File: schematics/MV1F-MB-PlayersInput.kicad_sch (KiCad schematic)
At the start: 55 parts

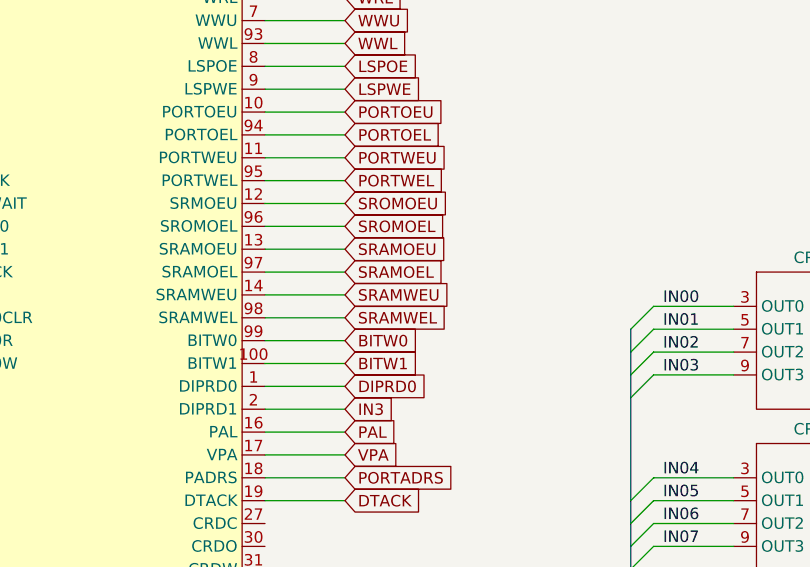
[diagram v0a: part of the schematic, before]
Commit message: Typo
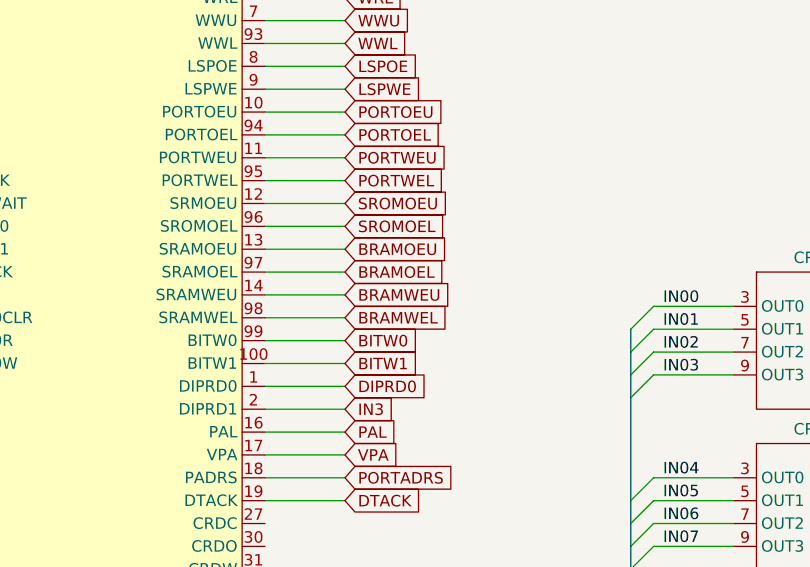
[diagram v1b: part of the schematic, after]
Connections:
- net SRAMOEL renamed BRAMOEL
- net SRAMOEU renamed BRAMOEU
- net SRAMWEL renamed BRAMWEL
- net SRAMWEU renamed BRAMWEU
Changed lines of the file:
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@@
     )
   )
-  (global_label "SRAMWEL" (shape input) (at 109.22 67.31 0) (fields_autoplaced)
-    (effects (font (size 1.27 1.27)) (justify left))
-    (property "Intersheetrefs" "${INTERSHEET_REFS}" (at 120.8532 67.31 0)
+  (global_label "BRAMWEL" (shape input) (at 109.22 67.31 0) (fields_autoplaced)
+    (effects (font (size 1.27 1.27)) (justify left))
+    (property "Intersheetrefs" "${INTERSHEET_REFS}" (at 120.9137 67.31 0)
       (effects (font (size 1.27 1.27)) (justify left))
     )
@@
     )
   )
-  (global_label "SRAMOEU" (shape input) (at 109.22 59.69 0) (fields_autoplaced)
-    (effects (font (size 1.27 1.27)) (justify left))
-    (property "Intersheetrefs" "${INTERSHEET_REFS}" (at 121.0347 59.69 0)
+  (global_label "BRAMOEU" (shape input) (at 109.22 59.69 0) (fields_autoplaced)
+    (effects (font (size 1.27 1.27)) (justify left))
+    (property "Intersheetrefs" "${INTERSHEET_REFS}" (at 121.0952 59.69 0)
       (effects (font (size 1.27 1.27)) (justify left))
     )
@@
     )
   )
-  (global_label "SRAMOEL" (shape input) (at 109.22 62.23 0) (fields_autoplaced)
-    (effects (font (size 1.27 1.27)) (justify left))
-    (property "Intersheetrefs" "${INTERSHEET_REFS}" (at 120.7323 62.23 0)
+  (global_label "BRAMOEL" (shape input) (at 109.22 62.23 0) (fields_autoplaced)
+    (effects (font (size 1.27 1.27)) (justify left))
+    (property "Intersheetrefs" "${INTERSHEET_REFS}" (at 120.7928 62.23 0)
       (effects (font (size 1.27 1.27)) (justify left))
     )
@@
     )
   )
-  (global_label "SRAMWEU" (shape input) (at 109.22 64.77 0) (fields_autoplaced)
-    (effects (font (size 1.27 1.27)) (justify left))
-    (property "Intersheetrefs" "${INTERSHEET_REFS}" (at 121.1556 64.77 0)
-      (effects (font (size 1.27 1.27)) (justify left))
-    )
+  (global_label "BRAMWEU" (shape input) (at 109.22 64.77 0) (fields_autoplaced)
+    (effects (font (size 1.27 1.27)) (justify left))
+    (property "Intersheetrefs" "${INTERSHEET_REFS}" (at 121.2161 64.77 0)
+      (effects (font (size 1.27 1.27)) (justify left))
+    )
